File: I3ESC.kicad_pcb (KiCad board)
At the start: 4 copper layers, 84 x 54 mm, 169 parts, among them J1 JST SR/SZ, J10 VIN_BARREL, J11 Barrel_Jack, J12 JST SR/SZ, J2 Screw_Terminal_01x02, J3 Screw_Terminal_01x02, J4 Screw_Terminal_01x02, J5 Conn_01x06, J6 Wireless Coil, J7 VIN_TERMINAL, J8 Conn_01x06, J9 JST SR/SZ, Q1 YJG150N03A, Q10 YJG150N03A, Q11 YJG150N03A, Q12 YJG150N03A, Q13 YJG150N03A, Q2 YJG150N03A, Q3 YJG150N03A, Q4 YJG150N03A, Q5 YJG150N03A, Q6 YJG150N03A, Q7 AO3401A, Q8 YJG150N03A, Q9 YJG150N03A, SW1 reset, U1 SY8113BADC, U10 USBLC6-2P6, U11 IP6826, U12 FD8288T (DRV8300), U13 Qwiic1, U2 FD8288T (DRV8300), U3 SPX3819M5-L-3-3, U7 STM32G431CBUx, U8 ABM3B-8.000MHZ, U9 USB_C_Receptacle

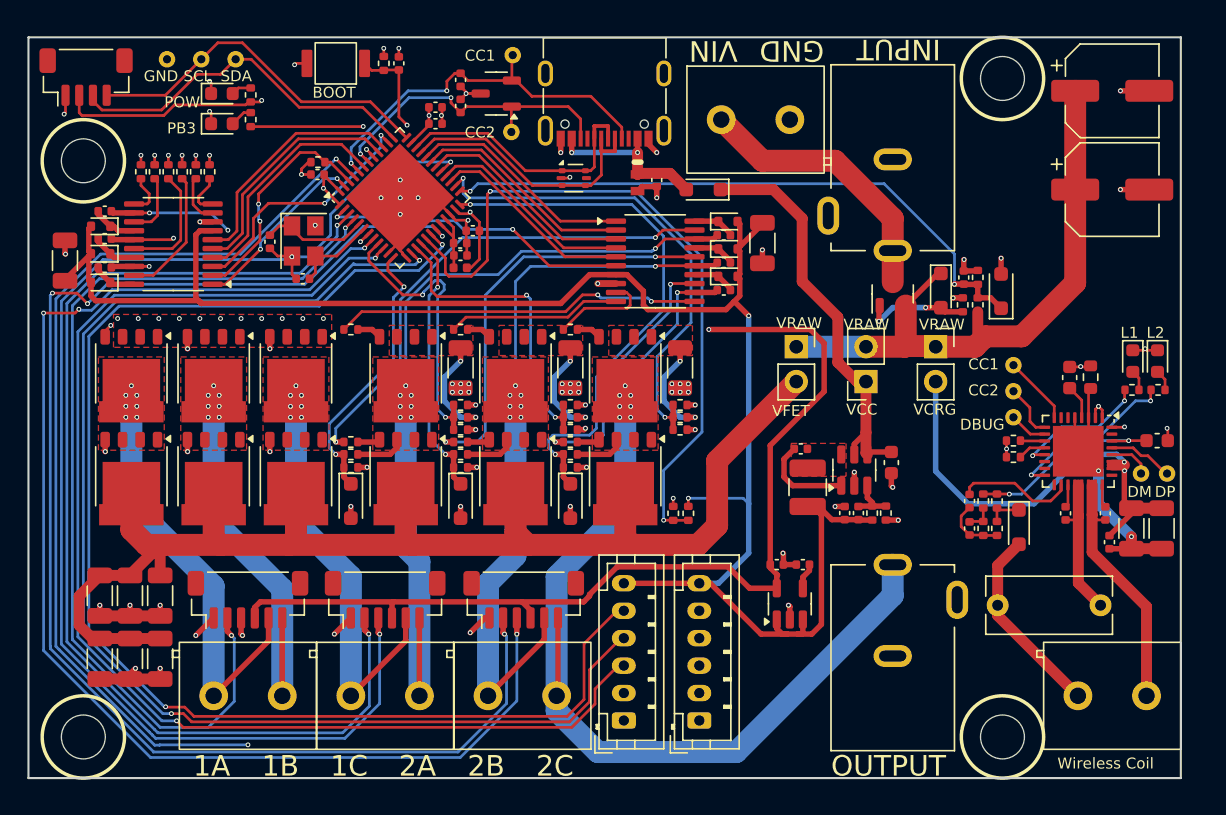
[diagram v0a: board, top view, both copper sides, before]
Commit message: first push for v2
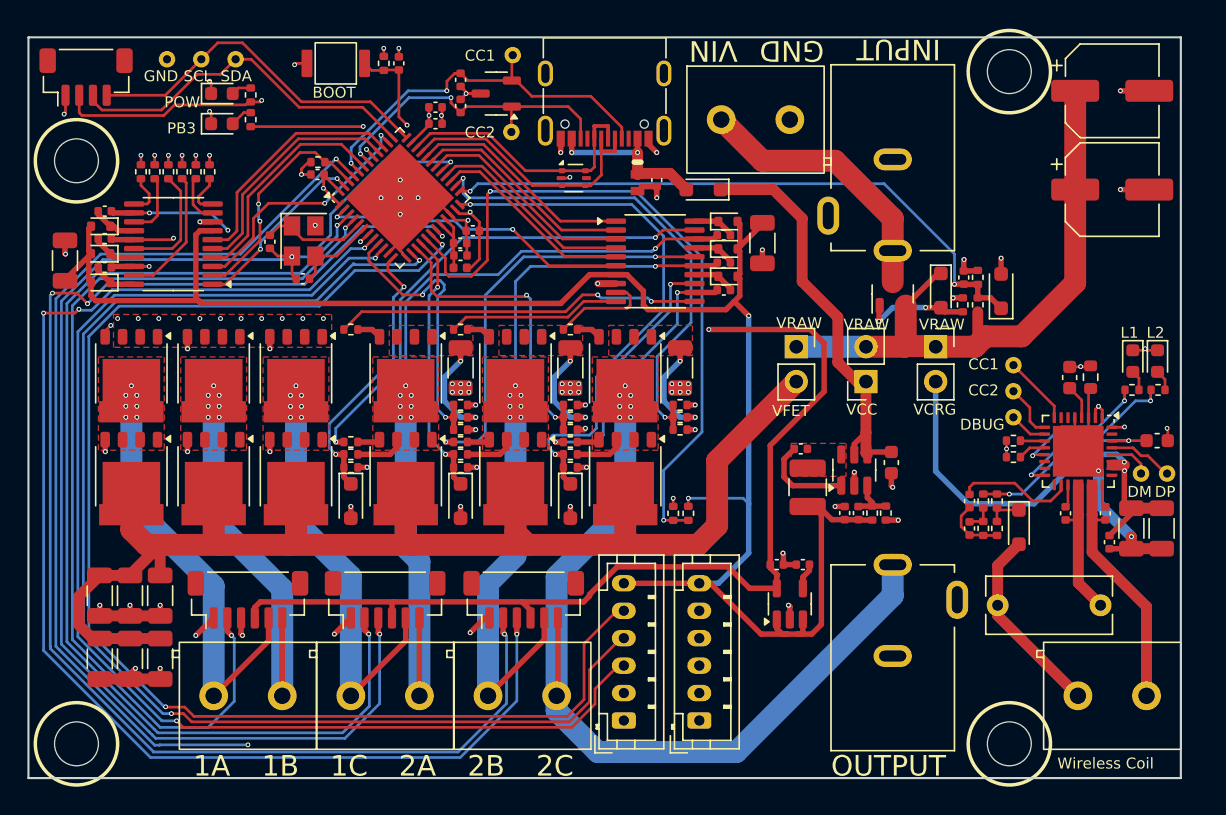
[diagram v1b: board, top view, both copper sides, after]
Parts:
- C1, C2, C3, C41, C43, C44: value 4.7uF,50V -> 4.7uF, 50V
- C10, C33, C34, C37: value 10uF,50V -> 10uF, 50V
- C13: value 2.2uF, 6.3V -> 2.2uF, 10V
- C15, C16: value 15pF -> 15pF, 50V
- C17, C27, C28, C32, C42, C900: value 100nF -> 100nF, 50V
- C20: value 2.2uF -> 2.2uF, 10V
- C22: value 10nF -> 10nF, 6.3V
- C29: value 250nF -> 250nF, 100V
- C35, C36: value 2.2uF -> 2.2uF, 50V
- C7, C8, C9: value 0.1uF -> 100nF, 50V
- moved H1 0.71 mm to (29.5, 24.5)
- moved H3 0.71 mm to (-38.5, 24.5)
- moved H4 0.71 mm to (29.5, -24.5)
- moved H2 0.50 mm to (-38.5, -18.0)
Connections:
- net S2_EN renamed Net-(U7-PG10)
- C31 pad 1: Net-(C31-Pad1) -> GND
- R34 pad 2: Net-(C31-Pad1) -> GND
- R35 pad 2: Net-(C31-Pad1) -> GND
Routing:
- net GND: track 89.7 -> 91.7 mm
- net Net-(C31-Pad1): track 1.99 -> 0.00 mm
